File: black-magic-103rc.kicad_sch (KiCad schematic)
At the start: 64 parts, among them J1 USB_B_Micro, J2 JTAG_SWD_10, J3 UART, J4 SWD_CONN, J5 BOOT0, Q1 DMG1024UV, Q2 DMG1023UV, SW1 SW_SPST, U1 USBLC6-2P6, U2 SN74LVC2T45DCUR, U3 STM32F103RCTx, U4 AMS1117-3.3, U5 SN74LVC2T45DCUR, U6 SN74LVC2T45DCUR, U7 SN74LVC2T45DCUR, Y2 8Mhz

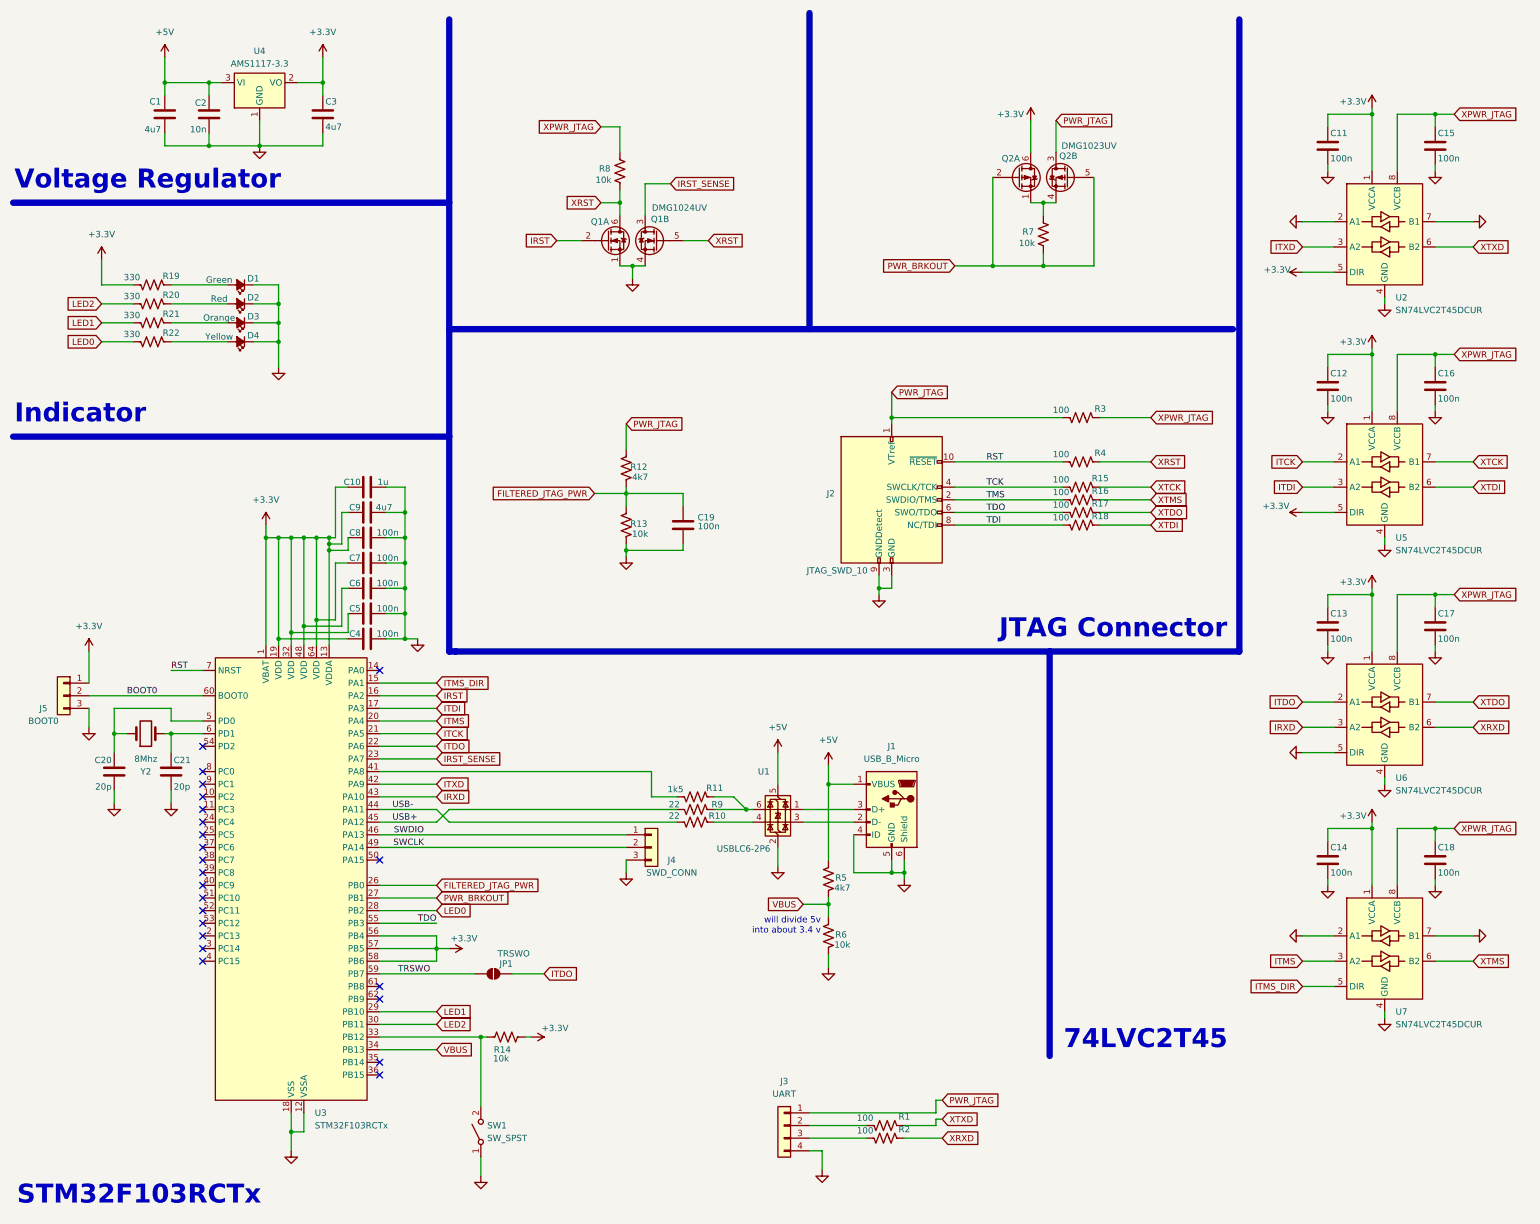
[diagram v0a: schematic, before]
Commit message: [02-04-1948] start to routing
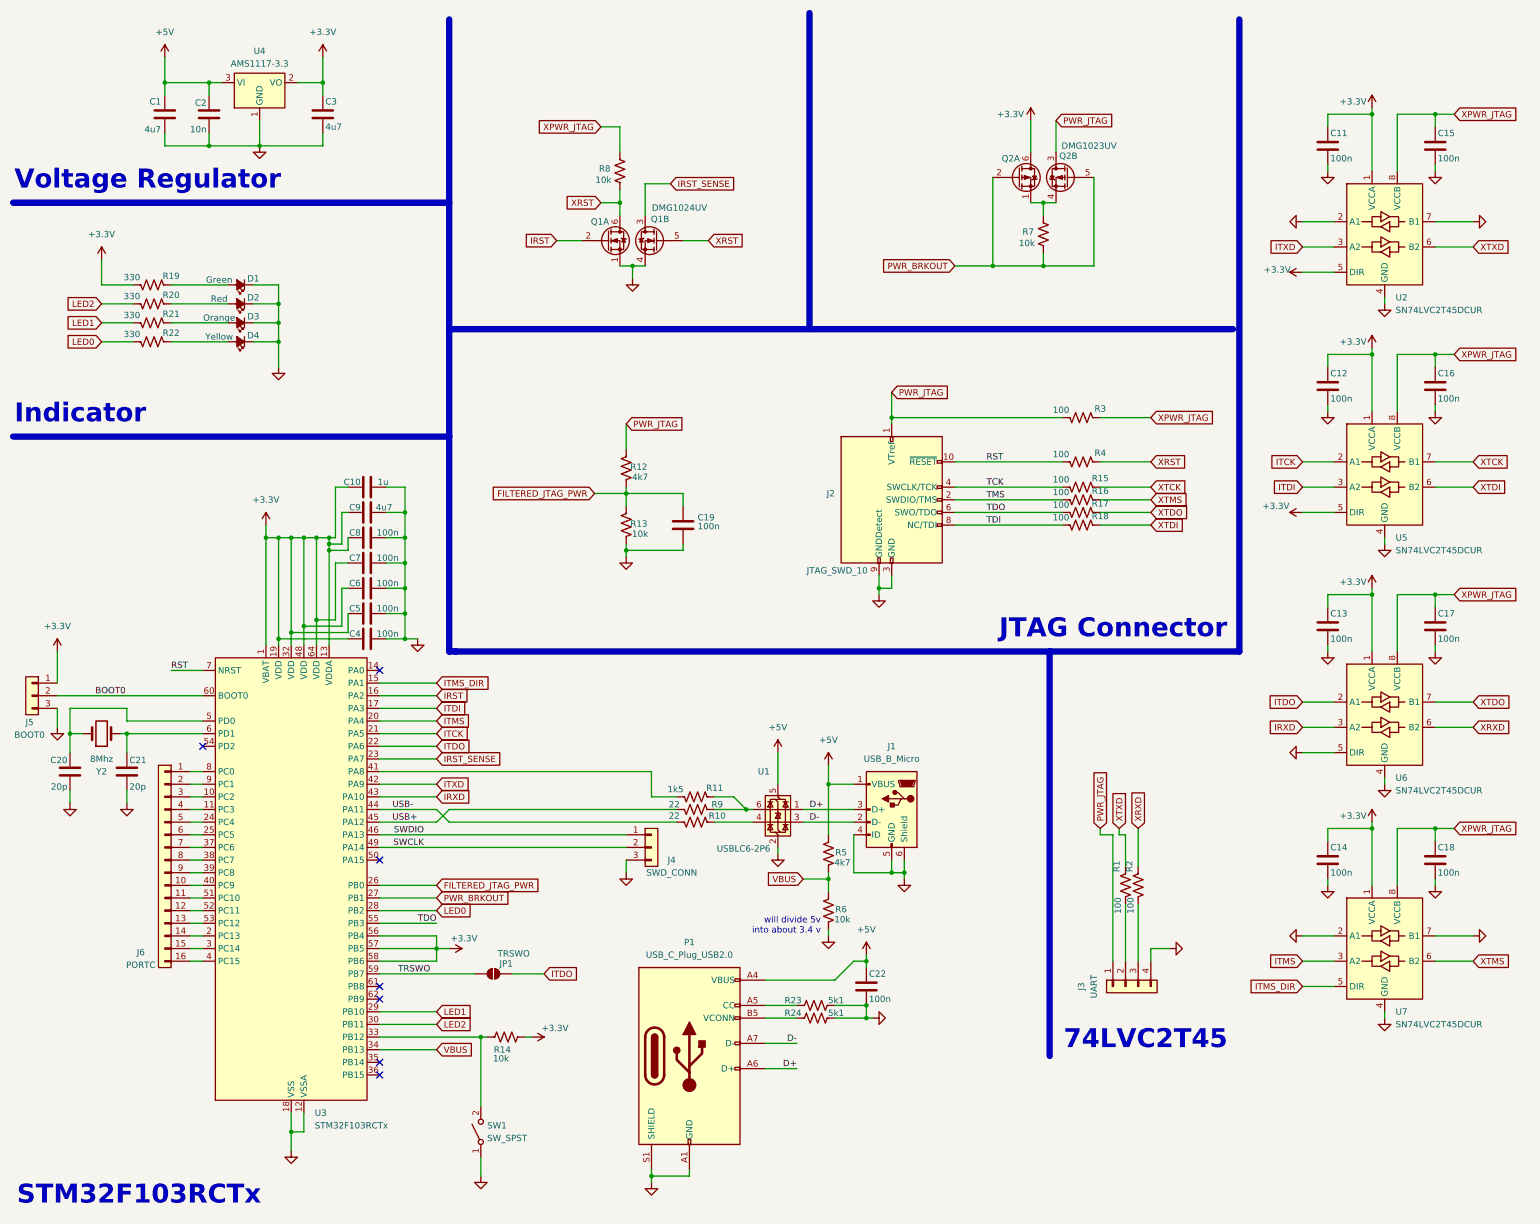
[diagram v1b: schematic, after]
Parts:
- added C22: 100n, Capacitor_SMD:C_0603_1608Metric_Pad1.08x0.95mm_HandSolder, symbol Device:C
- added J6: PORTC, Connector_PinHeader_1.27mm:PinHeader_1x16_P1.27mm_Horizontal, symbol Connector_Generic:Conn_01x16
- added P1: USB_C_Plug_USB2.0, Connector_USB:USB_C_Receptacle_GCT_USB4110, symbol Connector:USB_C_Plug_USB2.0
- added R23, R24: 5k1, Resistor_SMD:R_0805_2012Metric_Pad1.20x1.40mm_HandSolder, symbol Device:R_US
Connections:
- net +5V: now also C22.1, P1.A4 (VBUS), P1.A9 (VBUS), P1.B4 (VBUS), P1.B9 (VBUS)
- net GND: now also C22.2, P1.A1 (GND), P1.A12 (GND), P1.B1 (GND), P1.B12 (GND), P1.S1 (SHIELD), R23.1, R24.1
- net at U3.10 (PC2): now also J6.3 (Pin_3)
- net at U3.11 (PC3): now also J6.4 (Pin_4)
- net at U3.2 (PC13): now also J6.14 (Pin_14)
- net at U3.24 (PC4): now also J6.5 (Pin_5)
- net at U3.25 (PC5): now also J6.6 (Pin_6)
- net at U3.3 (PC14): now also J6.15 (Pin_15)
- net at U3.37 (PC6): now also J6.7 (Pin_7)
- net at U3.38 (PC7): now also J6.8 (Pin_8)
- net at U3.39 (PC8): now also J6.9 (Pin_9)
- net at U3.4 (PC15): now also J6.16 (Pin_16)
- net at U3.40 (PC9): now also J6.10 (Pin_10)
- net at U3.51 (PC10): now also J6.11 (Pin_11)
- net at U3.52 (PC11): now also J6.12 (Pin_12)
- net at U3.53 (PC12): now also J6.13 (Pin_13)
- net at U3.8 (PC0): now also J6.1 (Pin_1)
- net at U3.9 (PC1): now also J6.2 (Pin_2)
- net D+: now reaches J1.3 (D+), U1.1 (I/O1)
- net D+: now also P1.A6 (D+)
- net D-: now reaches J1.2 (D-), U1.3 (I/O2)
- net D-: now also P1.A7 (D-)
- new net: P1.A5 (CC), R23.2
- new net: P1.B5 (VCONN), R24.2
- no-connect marks 23 -> 7
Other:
- moved on the sheet: C20, C21, J3, J5, R1, R2, R5, R6, Y2

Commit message: [05-25-1348] generate bom
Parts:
- Q1, Q2: footprint Package_TO_SOT_SMD:SOT-363_SC-70-6_Handsoldering -> Package_TO_SOT_SMD:SOT-563
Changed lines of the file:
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@@
 			)
 		)
-		(property "Footprint" "Package_TO_SOT_SMD:SOT-363_SC-70-6_Handsoldering"
+		(property "Footprint" "Package_TO_SOT_SMD:SOT-563"
 			(at 217.17 45.72 0)
 			(effects
@@
 			)
 		)
-		(property "Footprint" "Package_TO_SOT_SMD:SOT-363_SC-70-6_Handsoldering"
+		(property "Footprint" "Package_TO_SOT_SMD:SOT-563"
 			(at 224.79 45.72 0)
 			(effects
@@
 			)
 		)
-		(property "Footprint" "Package_TO_SOT_SMD:SOT-363_SC-70-6_Handsoldering"
+		(property "Footprint" "Package_TO_SOT_SMD:SOT-563"
 			(at 138.43 58.42 0)
 			(effects
@@
 			)
 		)
-		(property "Footprint" "Package_TO_SOT_SMD:SOT-363_SC-70-6_Handsoldering"
+		(property "Footprint" "Package_TO_SOT_SMD:SOT-563"
 			(at 138.43 58.42 0)
 			(effects
